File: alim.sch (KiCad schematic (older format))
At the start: 18 parts, among them IC12 74LS139, IC2 74LS09, IC5 74LS123, IC6 74LS393, IC7 74LS14, IC8 74LS04, IC9 74LS11

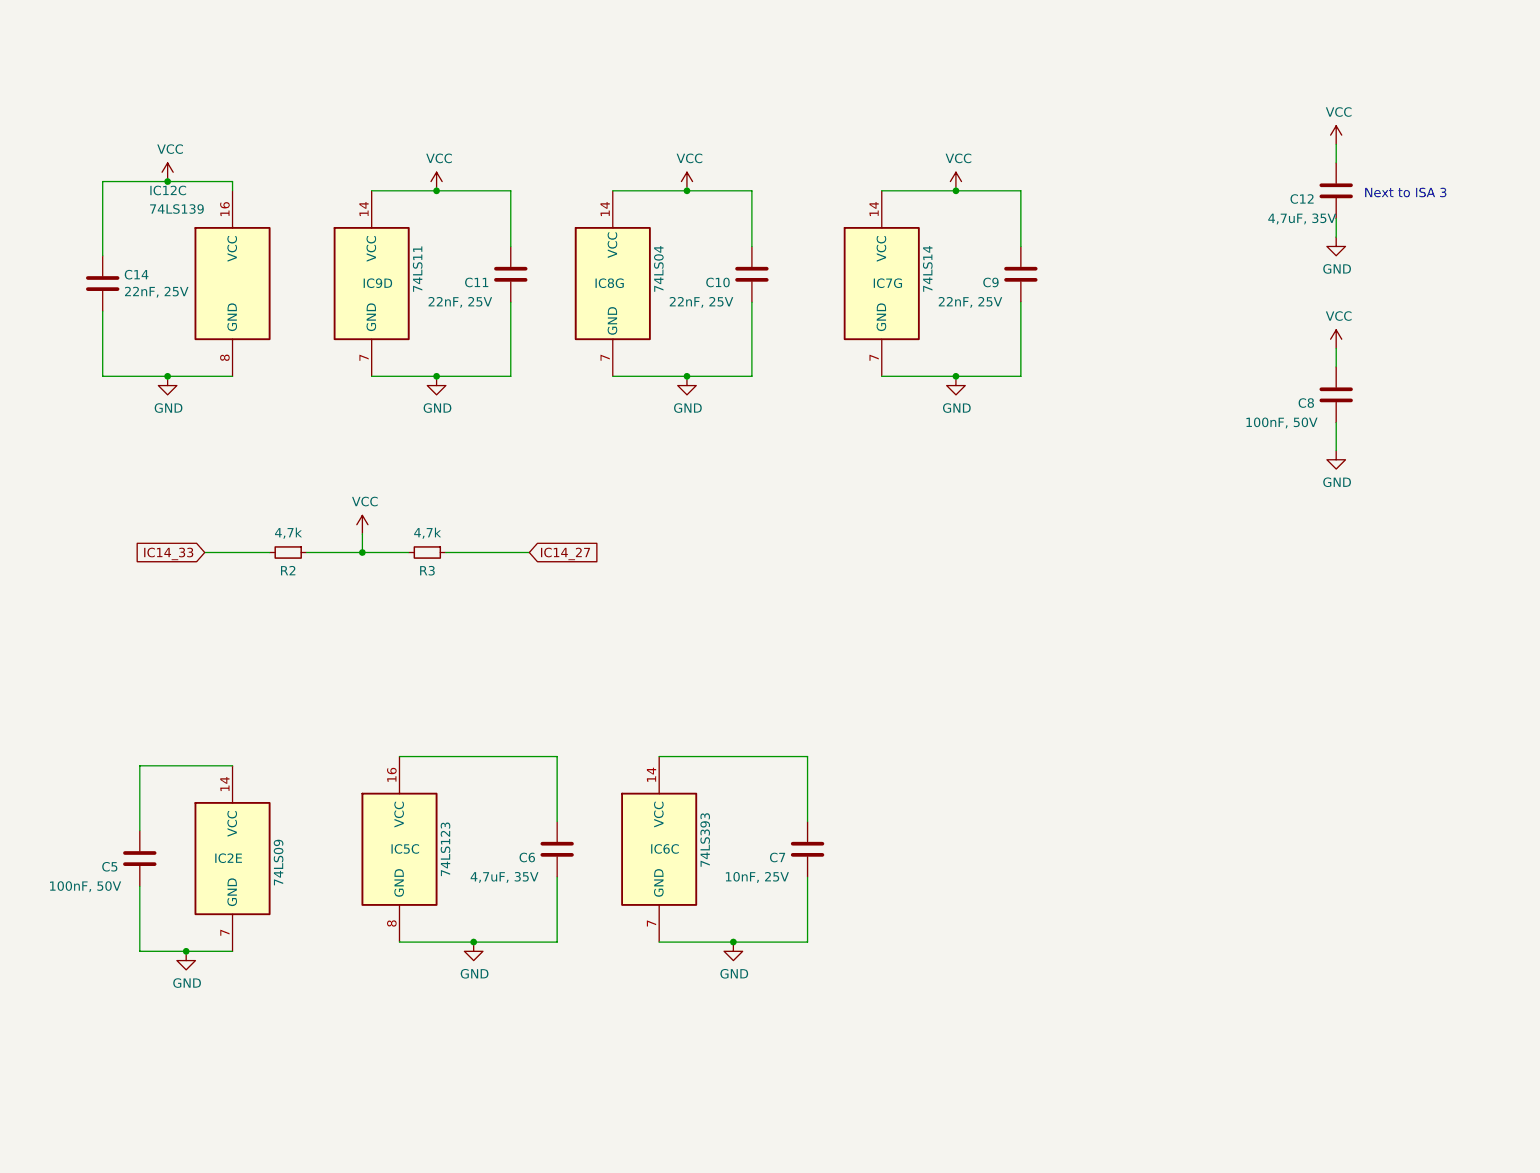
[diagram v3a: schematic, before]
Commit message: Maj de Freddy
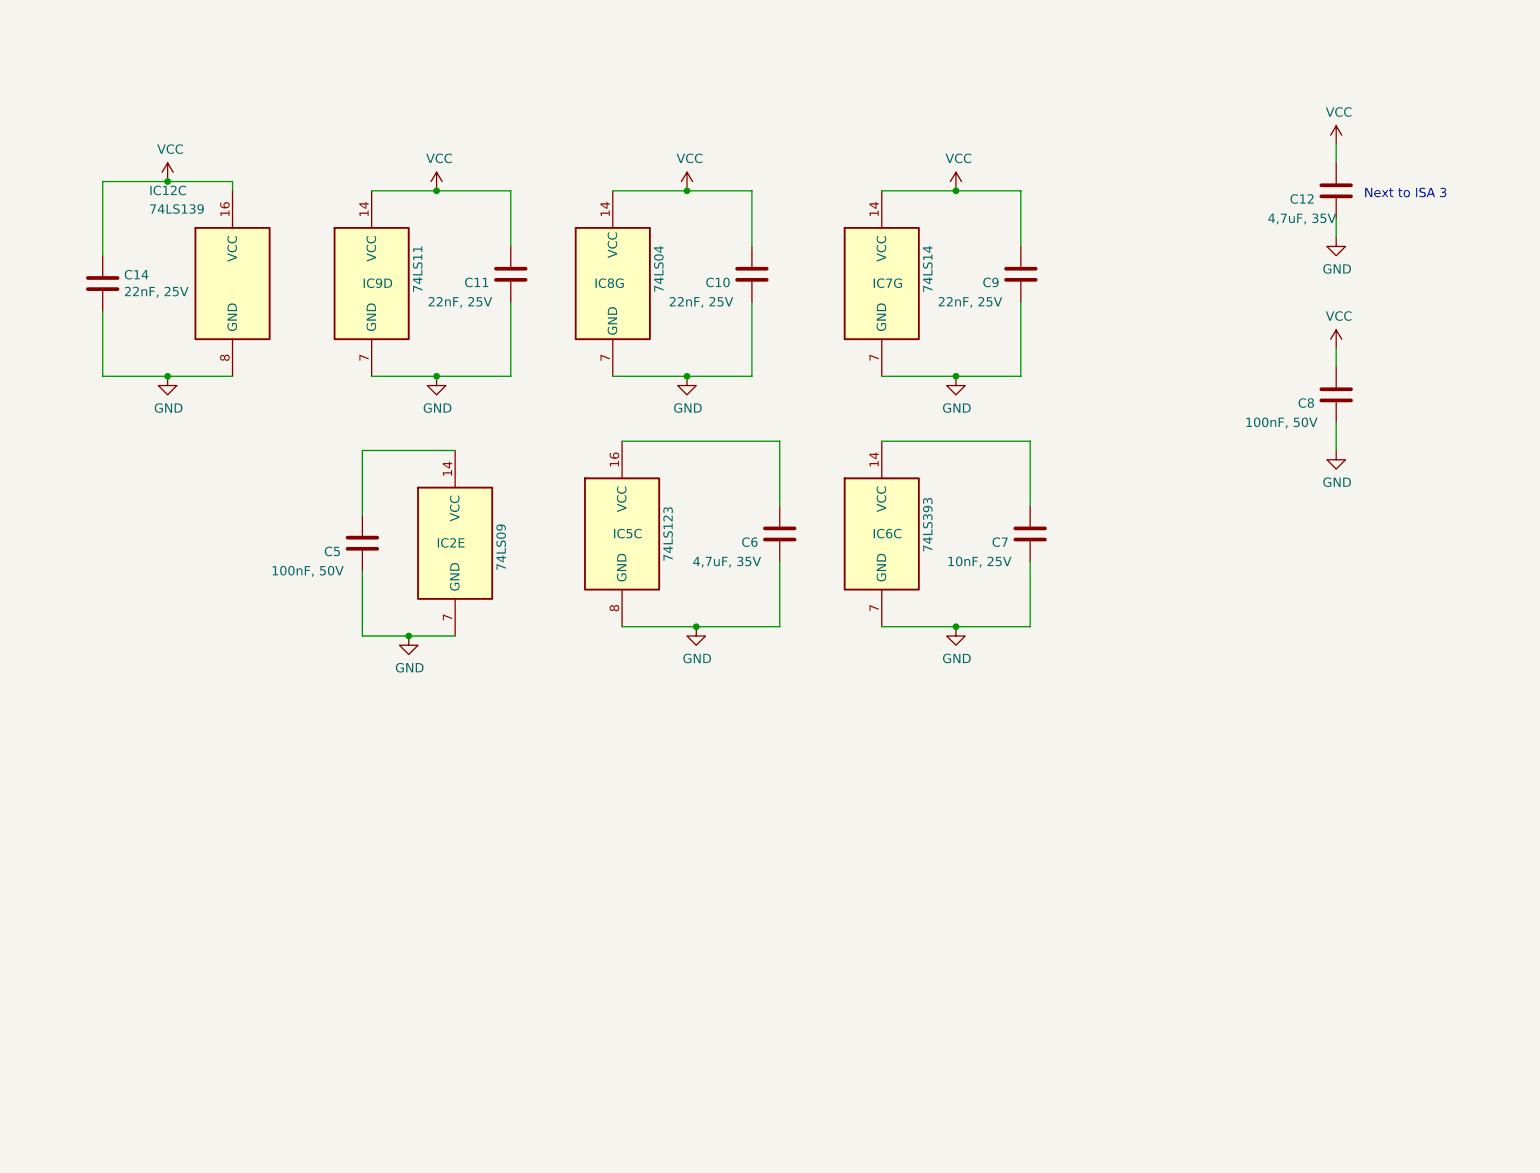
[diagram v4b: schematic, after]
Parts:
- removed R2, R3: 4,7k, Resistor_THT:R_Axial_DIN0309_L9.0mm_D3.2mm_P12.70mm_Horizontal, symbol Device:R_Small
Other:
- moved on the sheet: C5, C6, C7, IC2E, IC5C, IC6C
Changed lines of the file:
@@
 L Device:C C?
 U 1 1 61C0766A
-P 4650 5050
+P 5850 3350
 AR Path="/61C0766A" Ref="C?"  Part="1"
 AR Path="/6126F7E9/61C0766A" Ref="C?"  Part="1"
 AR Path="/61BDF4AD/61C0766A" Ref="C7"  Part="1"
-F 0 "C7" H 4765 5096 50  0000 L CNN
-F 1 "10nF, 25V" H 4750 5200 50  0000 L CNN
-F 2 "Capacitor_THT:C_Disc_D4.3mm_W1.9mm_P5.00mm" H 4688 4900 50  0001 C CNN
-F 3 "~" H 4650 5050 50  0001 C CNN
-	1    4650 5050
+F 0 "C7" H 5965 3396 50  0000 L CNN
+F 1 "10nF, 25V" H 5950 3500 50  0000 L CNN
+F 2 "Capacitor_THT:C_Disc_D4.3mm_W1.9mm_P5.00mm" H 5888 3200 50  0001 C CNN
+F 3 "~" H 5850 3350 50  0001 C CNN
+	1    5850 3350
 	-1   0    0    1
 $EndComp
@@
 L Device:C C?
 U 1 1 61C07688
-P 3300 5050
+P 4500 3350
 AR Path="/61C07688" Ref="C?"  Part="1"
 AR Path="/6126F7E9/61C07688" Ref="C?"  Part="1"
 AR Path="/61BDF4AD/61C07688" Ref="C6"  Part="1"
-F 0 "C6" H 3415 5096 50  0000 L CNN
-F 1 "4,7uF, 35V" H 3400 5200 50  0000 L CNN
-F 2 "Capacitor_THT:C_Disc_D4.3mm_W1.9mm_P5.00mm" H 3338 4900 50  0001 C CNN
-F 3 "~" H 3300 5050 50  0001 C CNN
-	1    3300 5050
+F 0 "C6" H 4615 3396 50  0000 L CNN
+F 1 "4,7uF, 35V" H 4600 3500 50  0000 L CNN
+F 2 "Capacitor_THT:C_Disc_D4.3mm_W1.9mm_P5.00mm" H 4538 3200 50  0001 C CNN
+F 3 "~" H 4500 3350 50  0001 C CNN
+	1    4500 3350
 	-1   0    0    1
 $EndComp
@@
 L 74xx:74LS393 IC?
 U 3 1 61C0768E
-P 3850 5050
+P 5050 3350
 AR Path="/61C0768E" Ref="IC?"  Part="3"
 AR Path="/6126F7E9/61C0768E" Ref="IC?"  Part="3"
 AR Path="/61BDF4AD/61C0768E" Ref="IC6"  Part="3"
-F 0 "IC6" H 3800 5050 50  0000 L CNN
-F 1 "74LS393" V 4100 4950 50  0000 L CNN
-F 2 "Package_DIP:DIP-14_W7.62mm" H 3850 5050 50  0001 C CNN
-F 3 "74xx\\74LS393.pdf" H 3850 5050 50  0001 C CNN
-	3    3850 5050
+F 0 "IC6" H 5000 3350 50  0000 L CNN
+F 1 "74LS393" V 5300 3250 50  0000 L CNN
+F 2 "Package_DIP:DIP-14_W7.62mm" H 5050 3350 50  0001 C CNN
+F 3 "74xx\\74LS393.pdf" H 5050 3350 50  0001 C CNN
+	3    5050 3350
 	1    0    0    -1
 $EndComp
@@
 L 74xx:74LS09 IC?
 U 5 1 61C07694
-P 1550 5100
+P 2750 3400
 AR Path="/61C07694" Ref="IC?"  Part="5"
 AR Path="/6126F7E9/61C07694" Ref="IC?"  Part="5"
 AR Path="/61BDF4AD/61C07694" Ref="IC2"  Part="5"
-F 0 "IC2" H 1450 5100 50  0000 L CNN
-F 1 "74LS09" V 1800 4950 50  0000 L CNN
-F 2 "Package_DIP:DIP-14_W7.62mm" H 1550 5100 50  0001 C CNN
-F 3 "http://www.ti.com/lit/gpn/sn74LS09" H 1550 5100 50  0001 C CNN
-	5    1550 5100
+F 0 "IC2" H 2650 3400 50  0000 L CNN
+F 1 "74LS09" V 3000 3250 50  0000 L CNN
+F 2 "Package_DIP:DIP-14_W7.62mm" H 2750 3400 50  0001 C CNN
+F 3 "http://www.ti.com/lit/gpn/sn74LS09" H 2750 3400 50  0001 C CNN
+	5    2750 3400
 	1    0    0    -1
 $EndComp
@@
 L Device:C C?
 U 1 1 61C0769A
-P 1050 5100
+P 2250 3400
 AR Path="/61C0769A" Ref="C?"  Part="1"
 AR Path="/6126F7E9/61C0769A" Ref="C?"  Part="1"
 AR Path="/61BDF4AD/61C0769A" Ref="C5"  Part="1"
-F 0 "C5" H 1165 5146 50  0000 L CNN
-F 1 "100nF, 50V" H 1150 5250 50  0000 L CNN
-F 2 "Resistor_THT:R_Axial_DIN0309_L9.0mm_D3.2mm_P12.70mm_Horizontal" H 1088 4950 50  0001 C CNN
-F 3 "~" H 1050 5100 50  0001 C CNN
-	1    1050 5100
+F 0 "C5" H 2365 3446 50  0000 L CNN
+F 1 "100nF, 50V" H 2350 3550 50  0000 L CNN
+F 2 "Resistor_THT:R_Axial_DIN0309_L9.0mm_D3.2mm_P12.70mm_Horizontal" H 2288 3250 50  0001 C CNN
+F 3 "~" H 2250 3400 50  0001 C CNN
+	1    2250 3400
 	-1   0    0    1
 $EndComp
@@
 L 74xx:74LS123 IC?
 U 3 1 61C076A6
-P 2450 5050
+P 3650 3350
 AR Path="/61C076A6" Ref="IC?"  Part="3"
 AR Path="/6126F7E9/61C076A6" Ref="IC?"  Part="3"
 AR Path="/61BDF4AD/61C076A6" Ref="IC5"  Part="3"
-F 0 "IC5" H 2400 5050 50  0000 L CNN
-F 1 "74LS123" V 2700 4900 50  0000 L CNN
-F 2 "Package_DIP:DIP-16_W7.62mm" H 2450 5050 50  0001 C CNN
-F 3 "http://www.ti.com/lit/gpn/sn74LS123" H 2450 5050 50  0001 C CNN
-	3    2450 5050
+F 0 "IC5" H 3600 3350 50  0000 L CNN
+F 1 "74LS123" V 3900 3200 50  0000 L CNN
+F 2 "Package_DIP:DIP-16_W7.62mm" H 3650 3350 50  0001 C CNN
+F 3 "http://www.ti.com/lit/gpn/sn74LS123" H 3650 3350 50  0001 C CNN
+	3    3650 3350
 	1    0    0    -1
 $EndComp
@@
 $EndComp
 Wire Wire Line
-	1550 5600 1300 5600
-Wire Wire Line
-	1550 4600 1050 4600
+	2750 3900 2500 3900
+Wire Wire Line
+	2750 2900 2250 2900
 Wire Wire Line
 	5050 1500 5450 1500
@@
 	5800 2500 5800 2100
 Wire Wire Line
-	4650 5200 4650 5550
-Wire Wire Line
-	3300 5200 3300 5550
-Wire Wire Line
-	3300 4900 3300 4550
-Wire Wire Line
-	4650 4900 4650 4550
-Wire Wire Line
-	3300 5550 2850 5550
-Wire Wire Line
-	3300 4550 2450 4550
-Wire Wire Line
-	1050 5250 1050 5600
+	5850 3500 5850 3850
+Wire Wire Line
+	4500 3500 4500 3850
+Wire Wire Line
+	4500 3200 4500 2850
+Wire Wire Line
+	5850 3200 5850 2850
+Wire Wire Line
+	4500 3850 4050 3850
+Wire Wire Line
+	4500 2850 3650 2850
+Wire Wire Line
+	2250 3550 2250 3900
 Wire Wire Line
 	3600 2500 4000 2500
@@
 Wire Wire Line
 	3050 1500 3050 1800
-$Comp
-L Device:R_Small R?
-U 1 1 6132D869
-P 2600 3450
-AR Path="/6126F7E9/6132D869" Ref="R?"  Part="1"
-AR Path="/61BDF4AD/6132D869" Ref="R3"  Part="1"
-F 0 "R3" V 2700 3450 50  0000 C CNN
-F 1 "4,7k" V 2495 3450 50  0000 C CNN
-F 2 "Resistor_THT:R_Axial_DIN0309_L9.0mm_D3.2mm_P12.70mm_Horizontal" H 2600 3450 50  0001 C CNN
-F 3 "~" H 2600 3450 50  0001 C CNN
-	1    2600 3450
-	0    1    1    0
-$EndComp
 $Comp
 L Device:C C?
@@
 $EndComp
 Wire Wire Line
-	3850 4550 4650 4550
-Wire Wire Line
-	3850 5550 4250 5550
+	5050 2850 5850 2850
+Wire Wire Line
+	5050 3850 5450 3850
 Wire Wire Line
 	2300 2500 2650 2500
 Wire Wire Line
 	2300 1500 2650 1500
-$Comp
-L Device:R_Small R?
-U 1 1 614CCF22
-P 1850 3450
-AR Path="/6126F7E9/614CCF22" Ref="R?"  Part="1"
-AR Path="/61BDF4AD/614CCF22" Ref="R2"  Part="1"
-F 0 "R2" V 1950 3450 50  0000 C CNN
-F 1 "4,7k" V 1745 3450 50  0000 C CNN
-F 2 "Resistor_THT:R_Axial_DIN0309_L9.0mm_D3.2mm_P12.70mm_Horizontal" H 1850 3450 50  0001 C CNN
-F 3 "~" H 1850 3450 50  0001 C CNN
-	1    1850 3450
-	0    1    1    0
-$EndComp
-Wire Wire Line
-	2500 3450 2250 3450
-Wire Wire Line
-	2250 3450 1950 3450
-Connection ~ 2250 3450
-Text GLabel 1400 3450 0    50   Input ~ 0
-IC14_33
-Wire Wire Line
-	1750 3450 1400 3450
 Wire Wire Line
 	850  2150 850  2500
 Wire Wire Line
 	850  2500 1200 2500
-$Comp
-L power:VCC #PWR?
-U 1 1 6134C22C
-P 2250 3350
-F 0 "#PWR?" H 2250 3200 50  0001 C CNN
-F 1 "VCC" H 2265 3523 50  0000 C CNN
-F 2 "" H 2250 3350 50  0001 C CNN
-F 3 "" H 2250 3350 50  0001 C CNN
-	1    2250 3350
-	1    0    0    -1
-$EndComp
-Wire Wire Line
-	2250 3350 2250 3450
-Text GLabel 3150 3450 2    50   Input ~ 0
-IC14_27
-Wire Wire Line
-	3150 3450 2700 3450
 Text Notes 7650 1550 0    50   ~ 0
 Next to ISA 3
@@
 $EndComp
 Wire Wire Line
-	1050 4600 1050 4950
+	2250 2900 2250 3250
 $Comp
 L power:GND #PWR?
 U 1 1 61460403
-P 1300 5600
-F 0 "#PWR?" H 1300 5350 50  0001 C CNN
-F 1 "GND" H 1305 5427 50  0000 C CNN
-F 2 "" H 1300 5600 50  0001 C CNN
-F 3 "" H 1300 5600 50  0001 C CNN
-	1    1300 5600
-	1    0    0    -1
-$EndComp
-Connection ~ 1300 5600
-Wire Wire Line
-	1300 5600 1050 5600
+P 2500 3900
+F 0 "#PWR?" H 2500 3650 50  0001 C CNN
+F 1 "GND" H 2505 3727 50  0000 C CNN
+F 2 "" H 2500 3900 50  0001 C CNN
+F 3 "" H 2500 3900 50  0001 C CNN
+	1    2500 3900
+	1    0    0    -1
+$EndComp
+Connection ~ 2500 3900
+Wire Wire Line
+	2500 3900 2250 3900
 Wire Wire Line
 	7500 1250 7500 1350
@@
 L power:GND #PWR?
 U 1 1 61484294
-P 2850 5550
-F 0 "#PWR?" H 2850 5300 50  0001 C CNN
-F 1 "GND" H 2855 5377 50  0000 C CNN
-F 2 "" H 2850 5550 50  0001 C CNN
-F 3 "" H 2850 5550 50  0001 C CNN
-	1    2850 5550
-	1    0    0    -1
-$EndComp
-Connection ~ 2850 5550
-Wire Wire Line
-	2850 5550 2450 5550
+P 4050 3850
+F 0 "#PWR?" H 4050 3600 50  0001 C CNN
+F 1 "GND" H 4055 3677 50  0000 C CNN
+F 2 "" H 4050 3850 50  0001 C CNN
+F 3 "" H 4050 3850 50  0001 C CNN
+	1    4050 3850
+	1    0    0    -1
+$EndComp
+Connection ~ 4050 3850
+Wire Wire Line
+	4050 3850 3650 3850
 $Comp
 L power:GND #PWR?
 U 1 1 61484CE1
-P 4250 5550
-F 0 "#PWR?" H 4250 5300 50  0001 C CNN
-F 1 "GND" H 4255 5377 50  0000 C CNN
-F 2 "" H 4250 5550 50  0001 C CNN
-F 3 "" H 4250 5550 50  0001 C CNN
-	1    4250 5550
-	1    0    0    -1
-$EndComp
-Connection ~ 4250 5550
-Wire Wire Line
-	4250 5550 4650 5550
+P 5450 3850
+F 0 "#PWR?" H 5450 3600 50  0001 C CNN
+F 1 "GND" H 5455 3677 50  0000 C CNN
+F 2 "" H 5450 3850 50  0001 C CNN
+F 3 "" H 5450 3850 50  0001 C CNN
+	1    5450 3850
+	1    0    0    -1
+$EndComp
+Connection ~ 5450 3850
+Wire Wire Line
+	5450 3850 5850 3850
 Wire Wire Line
 	5800 1500 5800 1800
